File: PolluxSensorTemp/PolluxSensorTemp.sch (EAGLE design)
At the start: 4 parts

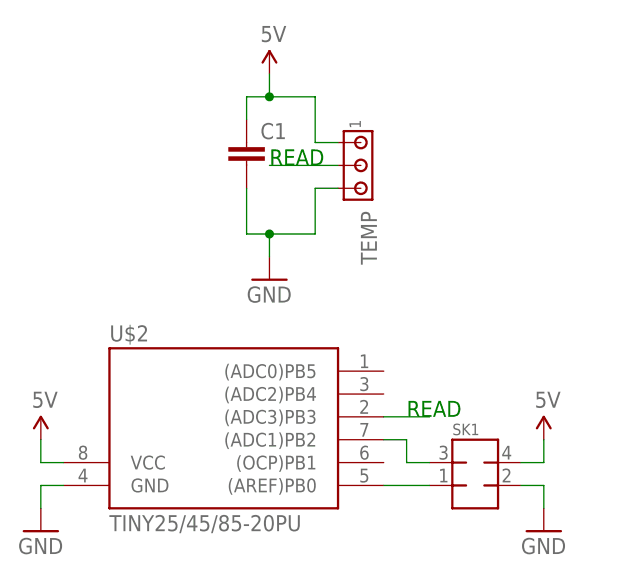
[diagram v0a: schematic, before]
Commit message: improve sensor board
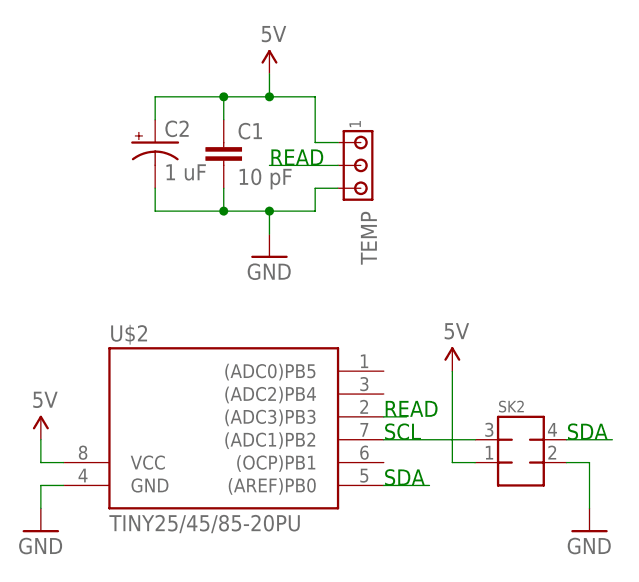
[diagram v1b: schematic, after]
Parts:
- removed SK1: (no value), jt-con-micromatch:MMATCH-8-PTH
- added C2: 1 uF, SparkFun:CAP_POLPTH2
- added SK2: (no value), jt-con-micromatch:MMATCH-8-PTH
- C1: value (none) -> 10 pF
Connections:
- removed net N$2: SK1.1, U$2.(AREF)PB0
- new net SDA: SK2.4, U$2.(AREF)PB0
- net 5V: now also C2.+, SK2.1; no longer SK1.4
- net GND: now also C2.-, SK2.2; no longer SK1.2
- net N$1: now also SK2.3; no longer SK1.3
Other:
- note added: "SCL"
- note added: "SDA"
- moved on the sheet: C1
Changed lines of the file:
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@@
 </classes>
 <parts>
-<part name="GND1" library="SparkFun" deviceset="GND" device=""/>
-<part name="SK1" library="jt-con-micromatch" deviceset="MMATCH-8-*" device="PTH"/>
 <part name="U$2" library="avr-7" deviceset="TINY25/45/85" device="-20PU"/>
 <part name="U$3" library="SparkFun" deviceset="5V" device=""/>
-<part name="U$4" library="SparkFun" deviceset="5V" device=""/>
 <part name="GND2" library="SparkFun" deviceset="GND" device=""/>
 <part name="TEMP" library="con-amp" deviceset="MTA03-100" device=""/>
-<part name="C1" library="SparkFun" deviceset="CAP" device="PTH1"/>
+<part name="C1" library="SparkFun" deviceset="CAP" device="PTH1" value="10 pF"/>
 <part name="U$1" library="SparkFun" deviceset="5V" device=""/>
 <part name="GND3" library="SparkFun" deviceset="GND" device=""/>
+<part name="SK2" library="jt-con-micromatch" deviceset="MMATCH-8-*" device="PTH"/>
+<part name="U$5" library="SparkFun" deviceset="5V" device=""/>
+<part name="GND4" library="SparkFun" deviceset="GND" device=""/>
+<part name="C2" library="SparkFun" deviceset="CAP_POL" device="PTH2" value="1 uF"/>
 </parts>
 <sheets>
@@
 <plain>
 <text x="58.42" y="58.42" size="1.778" layer="91">READ</text>
-<text x="73.66" y="30.48" size="1.778" layer="91">READ</text>
+<text x="71.12" y="30.48" size="1.778" layer="91">READ</text>
+<text x="71.12" y="27.94" size="1.778" layer="91">SCL</text>
+<text x="71.12" y="22.86" size="1.778" layer="91">SDA</text>
+<text x="91.44" y="27.94" size="1.778" layer="91">SDA</text>
 </plain>
 <instances>
-<instance part="GND1" gate="1" x="88.9" y="17.78"/>
-<instance part="SK1" gate="G$1" x="81.28" y="22.86"/>
 <instance part="U$2" gate="G$1" x="53.34" y="27.94"/>
 <instance part="U$3" gate="G$1" x="33.02" y="27.94"/>
-<instance part="U$4" gate="G$1" x="88.9" y="27.94"/>
 <instance part="GND2" gate="1" x="33.02" y="17.78"/>
 <instance part="TEMP" gate="G$1" x="68.58" y="58.42" rot="R270"/>
-<instance part="C1" gate="G$1" x="55.88" y="58.42"/>
+<instance part="C1" gate="G$1" x="53.34" y="58.42"/>
 <instance part="U$1" gate="G$1" x="58.42" y="68.58"/>
-<instance part="GND3" gate="1" x="58.42" y="45.72"/>
+<instance part="GND3" gate="1" x="58.42" y="48.26"/>
+<instance part="SK2" gate="G$1" x="86.36" y="25.4"/>
+<instance part="U$5" gate="G$1" x="78.74" y="35.56"/>
+<instance part="GND4" gate="1" x="93.98" y="17.78"/>
+<instance part="C2" gate="G$1" x="45.72" y="60.96"/>
 </instances>
 <busses>
 </busses>
 <nets>
-<net name="N$2" class="0">
-<segment>
-<pinref part="SK1" gate="G$1" pin="1"/>
-<pinref part="U$2" gate="G$1" pin="(AREF)PB0"/>
-<wire x1="76.2" y1="22.86" x2="71.12" y2="22.86" width="0.1524" layer="91"/>
-</segment>
-</net>
 <net name="5V" class="0">
-<segment>
-<pinref part="SK1" gate="G$1" pin="4"/>
-<wire x1="86.36" y1="25.4" x2="88.9" y2="25.4" width="0.1524" layer="91"/>
-<pinref part="U$4" gate="G$1" pin="5V"/>
-<wire x1="88.9" y1="25.4" x2="88.9" y2="27.94" width="0.1524" layer="91"/>
-</segment>
 <segment>
 <pinref part="U$2" gate="G$1" pin="VCC"/>
@@
 <segment>
 <pinref part="C1" gate="G$1" pin="1"/>
-<wire x1="55.88" y1="63.5" x2="55.88" y2="66.04" width="0.1524" layer="91"/>
-<wire x1="55.88" y1="66.04" x2="58.42" y2="66.04" width="0.1524" layer="91"/>
+<wire x1="53.34" y1="63.5" x2="53.34" y2="66.04" width="0.1524" layer="91"/>
+<wire x1="53.34" y1="66.04" x2="58.42" y2="66.04" width="0.1524" layer="91"/>
 <wire x1="58.42" y1="66.04" x2="63.5" y2="66.04" width="0.1524" layer="91"/>
 <wire x1="63.5" y1="66.04" x2="63.5" y2="60.96" width="0.1524" layer="91"/>
@@
 <wire x1="58.42" y1="68.58" x2="58.42" y2="66.04" width="0.1524" layer="91"/>
 <junction x="58.42" y="66.04"/>
+<pinref part="C2" gate="G$1" pin="+"/>
+<wire x1="45.72" y1="63.5" x2="45.72" y2="66.04" width="0.1524" layer="91"/>
+<wire x1="45.72" y1="66.04" x2="53.34" y2="66.04" width="0.1524" layer="91"/>
+<junction x="53.34" y="66.04"/>
+</segment>
+<segment>
+<pinref part="SK2" gate="G$1" pin="1"/>
+<pinref part="U$5" gate="G$1" pin="5V"/>
+<wire x1="81.28" y1="25.4" x2="78.74" y2="25.4" width="0.1524" layer="91"/>
+<wire x1="78.74" y1="25.4" x2="78.74" y2="35.56" width="0.1524" layer="91"/>
 </segment>
 </net>
@@
 </segment>
 <segment>
-<pinref part="SK1" gate="G$1" pin="2"/>
-<wire x1="86.36" y1="22.86" x2="88.9" y2="22.86" width="0.1524" layer="91"/>
-<pinref part="GND1" gate="1" pin="GND"/>
-<wire x1="88.9" y1="22.86" x2="88.9" y2="20.32" width="0.1524" layer="91"/>
-</segment>
-<segment>
-<wire x1="58.42" y1="50.8" x2="63.5" y2="50.8" width="0.1524" layer="91"/>
-<wire x1="63.5" y1="50.8" x2="63.5" y2="55.88" width="0.1524" layer="91"/>
+<wire x1="58.42" y1="53.34" x2="63.5" y2="53.34" width="0.1524" layer="91"/>
+<wire x1="63.5" y1="53.34" x2="63.5" y2="55.88" width="0.1524" layer="91"/>
 <pinref part="TEMP" gate="G$1" pin="3"/>
 <wire x1="63.5" y1="55.88" x2="66.04" y2="55.88" width="0.1524" layer="91"/>
 <pinref part="GND3" gate="1" pin="GND"/>
-<wire x1="58.42" y1="48.26" x2="58.42" y2="50.8" width="0.1524" layer="91"/>
+<wire x1="58.42" y1="50.8" x2="58.42" y2="53.34" width="0.1524" layer="91"/>
 <pinref part="C1" gate="G$1" pin="2"/>
-<wire x1="55.88" y1="55.88" x2="55.88" y2="50.8" width="0.1524" layer="91"/>
-<wire x1="55.88" y1="50.8" x2="58.42" y2="50.8" width="0.1524" layer="91"/>
-<junction x="58.42" y="50.8"/>
+<wire x1="53.34" y1="55.88" x2="53.34" y2="53.34" width="0.1524" layer="91"/>
+<wire x1="53.34" y1="53.34" x2="58.42" y2="53.34" width="0.1524" layer="91"/>
+<junction x="58.42" y="53.34"/>
+<pinref part="C2" gate="G$1" pin="-"/>
+<wire x1="53.34" y1="53.34" x2="45.72" y2="53.34" width="0.1524" layer="91"/>
+<wire x1="45.72" y1="53.34" x2="45.72" y2="55.88" width="0.1524" layer="91"/>
+<junction x="53.34" y="53.34"/>
+</segment>
+<segment>
+<pinref part="SK2" gate="G$1" pin="2"/>
+<pinref part="GND4" gate="1" pin="GND"/>
+<wire x1="91.44" y1="25.4" x2="93.98" y2="25.4" width="0.1524" layer="91"/>
+<wire x1="93.98" y1="25.4" x2="93.98" y2="20.32" width="0.1524" layer="91"/>
 </segment>
 </net>
@@
 <segment>
 <pinref part="U$2" gate="G$1" pin="(ADC1)PB2"/>
-<wire x1="71.12" y1="27.94" x2="73.66" y2="27.94" width="0.1524" layer="91"/>
-<wire x1="73.66" y1="27.94" x2="73.66" y2="25.4" width="0.1524" layer="91"/>
-<pinref part="SK1" gate="G$1" pin="3"/>
-<wire x1="73.66" y1="25.4" x2="76.2" y2="25.4" width="0.1524" layer="91"/>
+<pinref part="SK2" gate="G$1" pin="3"/>
+<wire x1="71.12" y1="27.94" x2="81.28" y2="27.94" width="0.1524" layer="91"/>
 </segment>
 </net>
@@
 <segment>
 <pinref part="U$2" gate="G$1" pin="(ADC3)PB3"/>
-<wire x1="71.12" y1="30.48" x2="76.2" y2="30.48" width="0.1524" layer="91"/>
+<wire x1="71.12" y1="30.48" x2="73.66" y2="30.48" width="0.1524" layer="91"/>
 </segment>
 <segment>
@@
 </segment>
 </net>
+<net name="SDA" class="0">
+<segment>
+<pinref part="U$2" gate="G$1" pin="(AREF)PB0"/>
+<wire x1="76.2" y1="22.86" x2="71.12" y2="22.86" width="0.1524" layer="91"/>
+</segment>
+<segment>
+<pinref part="SK2" gate="G$1" pin="4"/>
+<wire x1="91.44" y1="27.94" x2="96.52" y2="27.94" width="0.1524" layer="91"/>
+</segment>
+</net>
